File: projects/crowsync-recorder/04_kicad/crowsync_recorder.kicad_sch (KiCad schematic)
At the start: 51 parts, among them J1 USB4105-GF-A, J2 JST-GH mic, J3 JST-GH PPS, U1 PCM2900CDBR, U2 TLV9062IDR, U3 TPS7A2033PDBVR, Y1 12MHz 3225 20pF

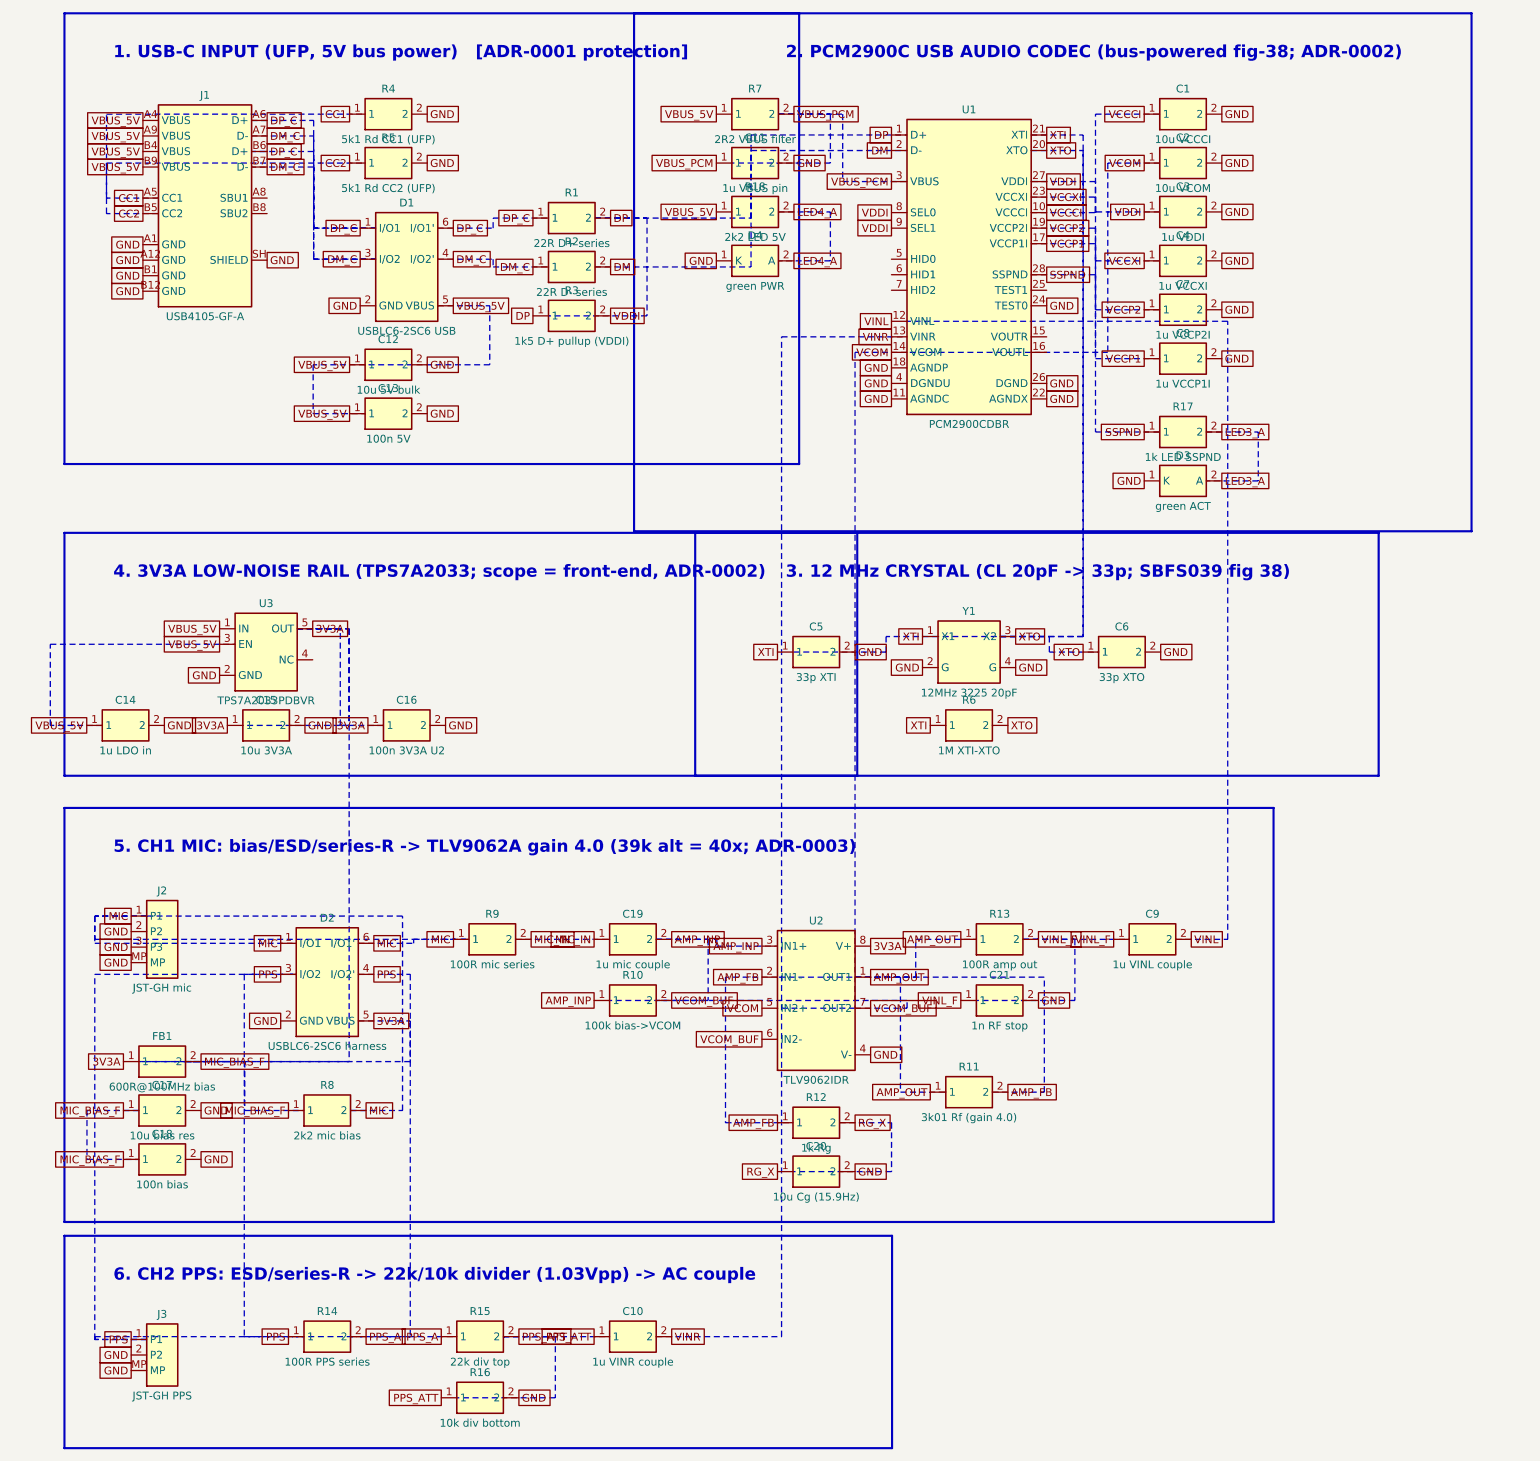
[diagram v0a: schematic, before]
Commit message: crowsync-recorder: schematic legibility fixes (render review triage), acceptance criteria met — design state for v1.0 release
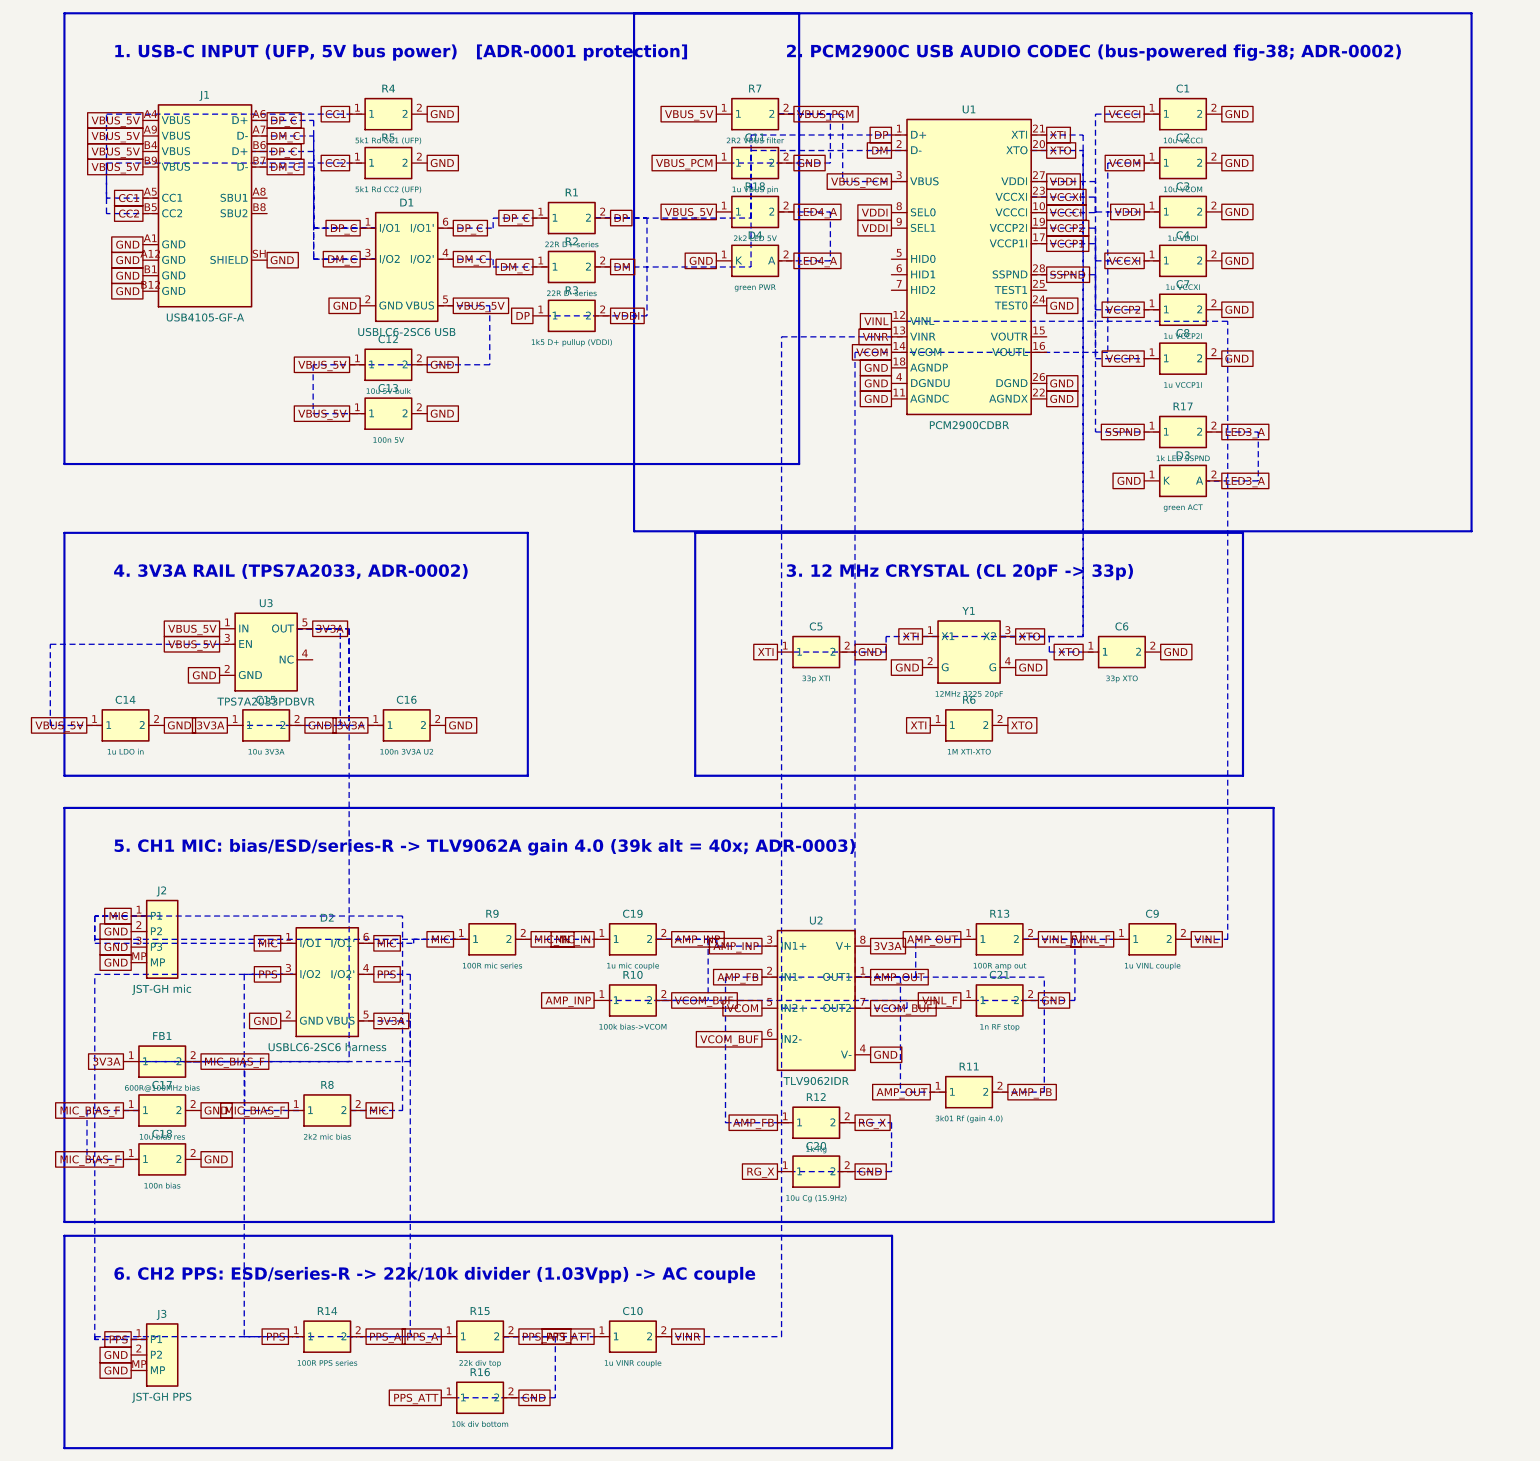
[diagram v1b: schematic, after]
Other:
- note added: "3. 12 MHz CRYSTAL (CL 20pF -> 33p)"
- note added: "4. 3V3A RAIL (TPS7A2033, ADR-0002)"
- note removed: "3. 12 MHz CRYSTAL (CL 20pF -> 33p; SBFS039 fig 38)"
- note removed: "4. 3V3A LOW-NOISE RAIL (TPS7A2033; scope = front-end, ADR-0002)"
